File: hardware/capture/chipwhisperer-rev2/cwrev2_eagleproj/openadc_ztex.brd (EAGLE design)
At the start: 155 x 100.3 mm, 219 parts, among them CON3 JTAG, CON6 USB-FPGA1.15, IC1 AOZ1021, IC2 AOZ1021, IC3 AOZ1094, IC5 AT90USB162A, T1 TC1-1T, U1 AD9215BRUZ, U10 ATSHA204-SH, U2 AD8331, U3 LP3985IM5-3.0, U4 LTC3200ES6, U5 CDCE906PW, U6 TXS0104EPWR, U7 TXB0108PWR, U8 SN74LVC1T45DBVT, U9 SN74LVC1T45DBVT, X1 SMA-142-0711-821/826, X2 SMA-142-0711-821/826, X3 SMA-142-0711-821/826, X4 SMA-142-0711-821/826, X5 PN61729-S

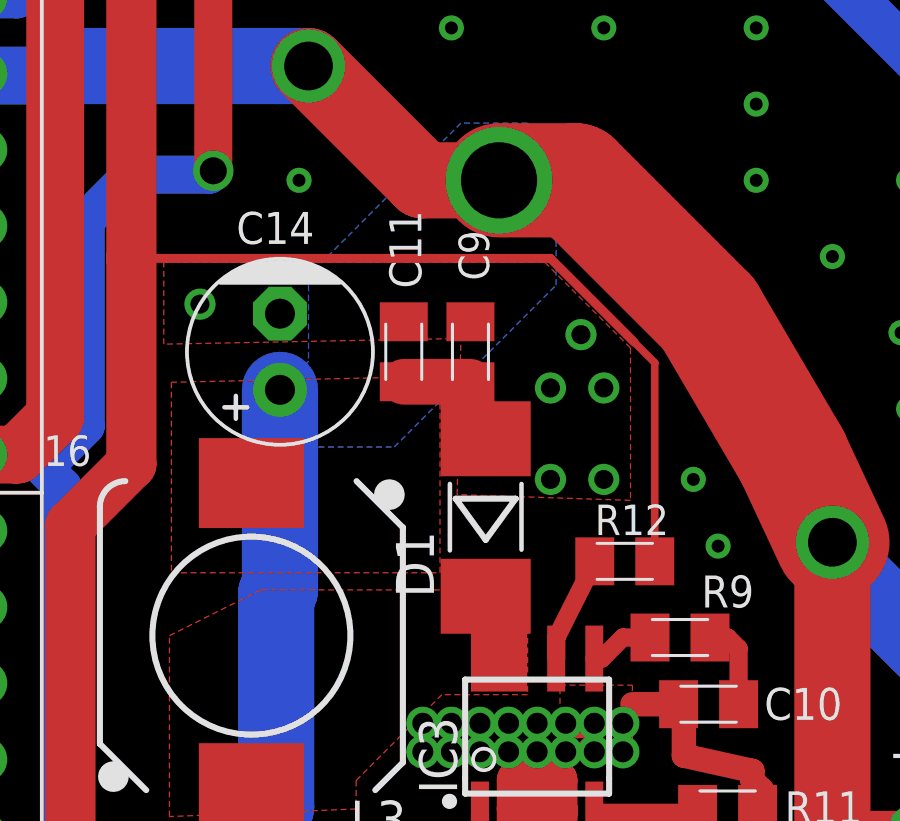
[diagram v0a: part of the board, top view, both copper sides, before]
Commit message: fix issue w/ CW Short on 1.2V rail
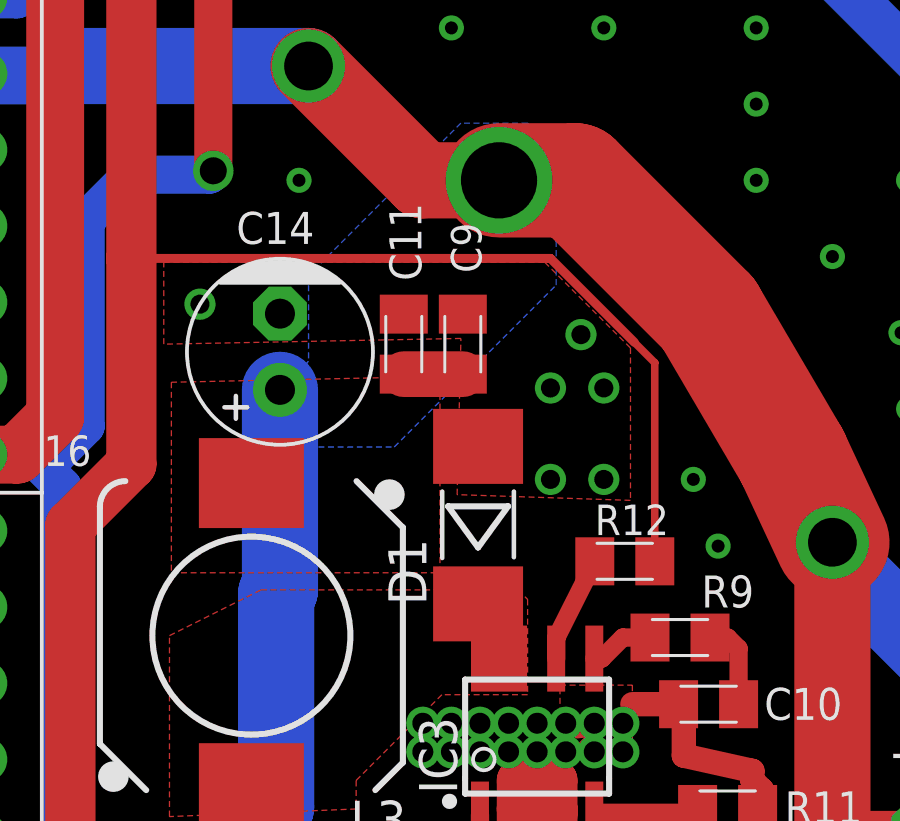
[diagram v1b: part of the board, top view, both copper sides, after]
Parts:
- moved C9 0.36 mm to (74.0, 58.4)
- moved D1 0.36 mm to (74.5, 52.3)
- moved C11 0.25 mm to (72.1, 58.4)
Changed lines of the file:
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@@
 <attribute name="VALUE" x="90.7465" y="96.631" size="1.0668" layer="27" ratio="12" rot="R270"/>
 </element>
-<element name="C11" library="myrcl" package="C0805K" value="22µ" x="72.0725" y="58.1025" smashed="yes" rot="R270">
-<attribute name="NAME" x="72.658" y="60.214" size="1.0668" layer="25" ratio="12" rot="R90"/>
-<attribute name="VALUE" x="70.988" y="56.404" size="1.0668" layer="27" ratio="12" rot="R90"/>
+<element name="C11" library="myrcl" package="C0805K" value="22µ" x="72.0725" y="58.3565" smashed="yes" rot="R270">
+<attribute name="NAME" x="72.658" y="60.468" size="1.0668" layer="25" ratio="12" rot="R90"/>
+<attribute name="VALUE" x="70.988" y="56.658" size="1.0668" layer="27" ratio="12" rot="R90"/>
 </element>
 <element name="R10" library="myrcl" package="R0805K" value="1K2" x="82.8675" y="39.6875" smashed="yes">
@@
 <attribute name="MPN" value="CDRH104RNP-2R5NC" x="66.9925" y="48.641" size="1.778" layer="27" rot="R180" display="off"/>
 </element>
-<element name="C9" library="myrcl" package="C0805K" value="22µ" x="74.295" y="58.1025" smashed="yes" rot="R270">
-<attribute name="NAME" x="73.9" y="62.1505" size="1.016" layer="25" rot="R270"/>
-<attribute name="VALUE" x="72.395" y="59.1025" size="1.016" layer="27" rot="R270"/>
-</element>
-<element name="D1" library="diode" package="MELF-MLL41" value="" x="74.803" y="52.578" rot="R90"/>
+<element name="C9" library="myrcl" package="C0805K" value="22µ" x="74.041" y="58.3565" smashed="yes" rot="R270">
+<attribute name="NAME" x="73.646" y="62.4045" size="1.016" layer="25" rot="R270"/>
+<attribute name="VALUE" x="72.141" y="59.3565" size="1.016" layer="27" rot="R270"/>
+</element>
+<element name="D1" library="diode" package="MELF-MLL41" value="" x="74.549" y="52.324" rot="R90"/>
 <element name="JP1" library="pinhead" package="1X02" value="" x="91.44" y="95.5675"/>
 <element name="U$3" library="openadc_footprint" package="OPENADCREV1" value="OPENADC" x="113.3475" y="77.1525" rot="R180"/>
@@
 <contactref element="CON6" pad="D28"/>
 <contactref element="CON6" pad="C28"/>
-<wire x1="74.295" y1="57.1025" x2="72.0725" y2="57.1025" width="1.524" layer="1"/>
+<wire x1="74.041" y1="57.3565" x2="72.0725" y2="57.3565" width="1.524" layer="1"/>
 <contactref element="TP4" pad="TP"/>
 <wire x1="89.408" y1="42.164" x2="86.614" y2="42.164" width="1.27" layer="1"/>
